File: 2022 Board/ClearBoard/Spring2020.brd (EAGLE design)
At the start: 100 x 80 mm, 18 parts, among them U1 TB67H401FTG(O,EL), U2 ABX00012, U3 V36SE05010NRFA

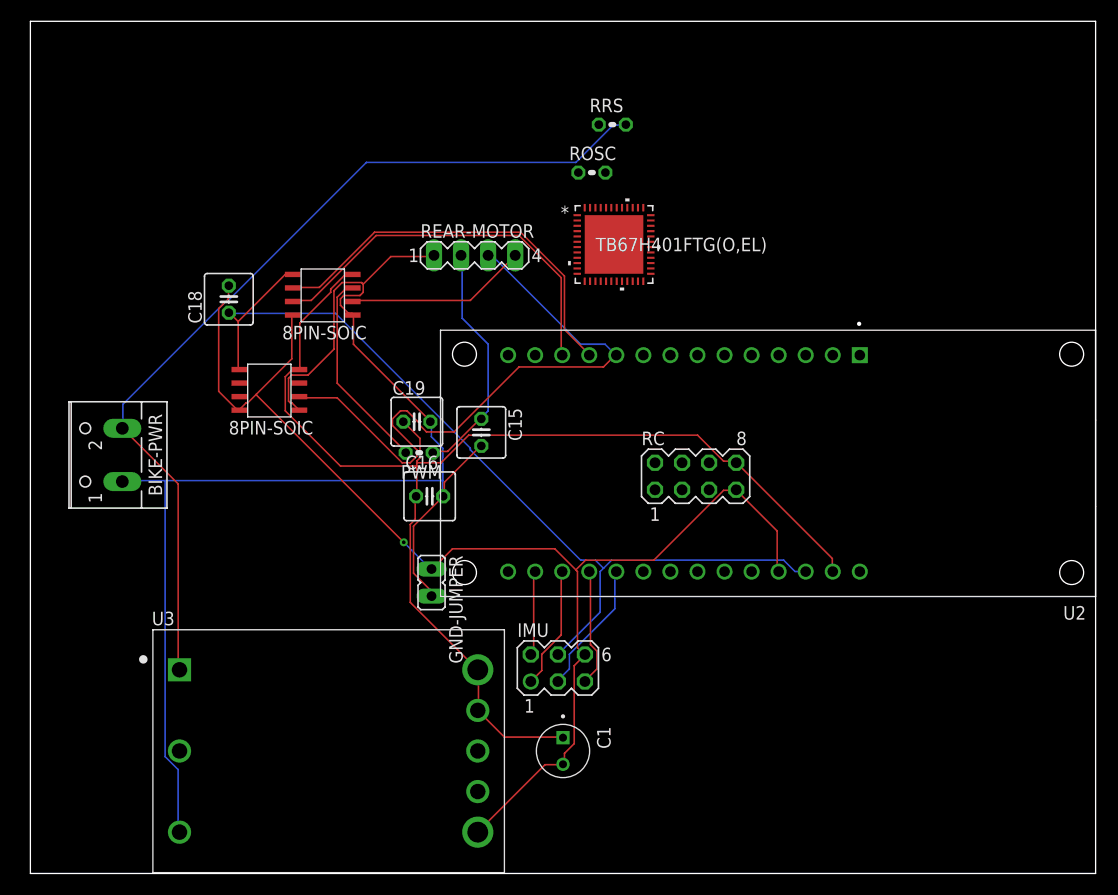
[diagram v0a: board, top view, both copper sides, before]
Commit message: Fixed a bunch of stuff
Routed most of the board
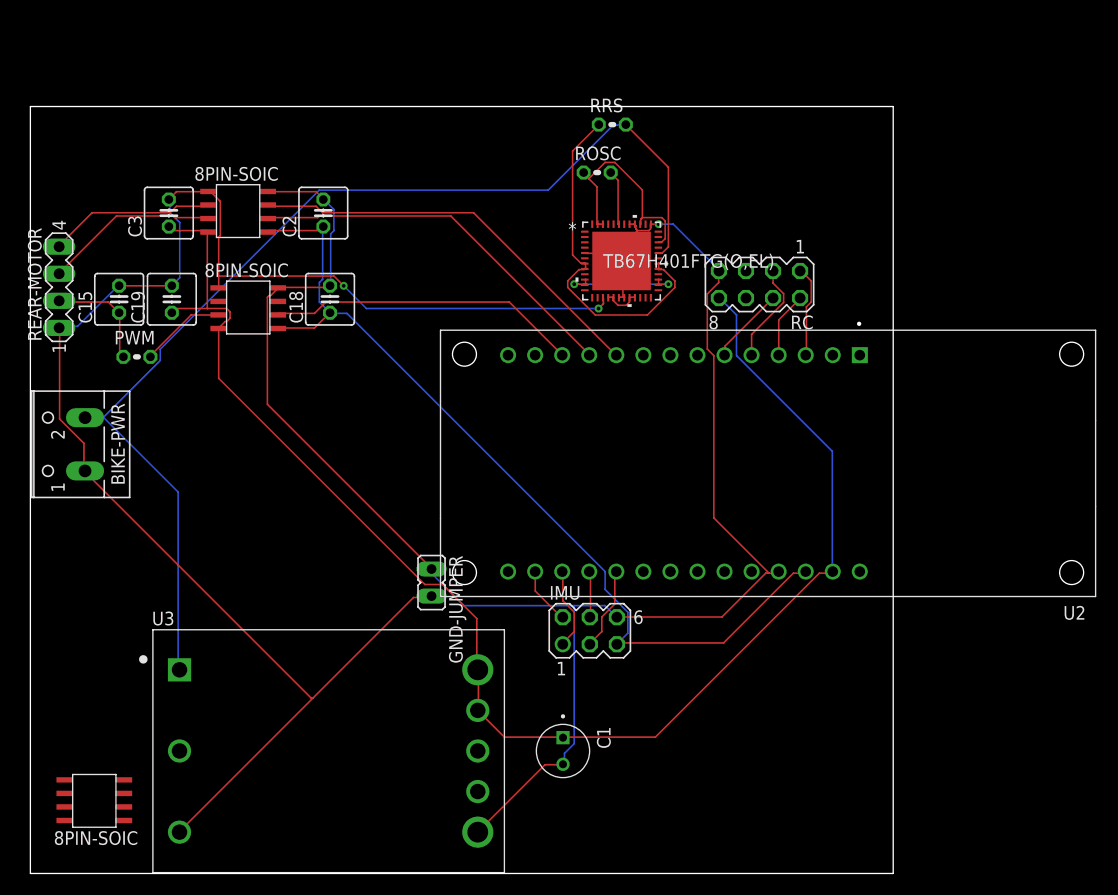
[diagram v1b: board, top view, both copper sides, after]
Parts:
- removed C16: (no value), resistor:C025-050X050
- added C2, C3: (no value), resistor:C025-050X050
- added U$3: IL-711, Spring2016Optoisolator:8PINSOIC
- U$2: value IL-711 -> IL-712
- U1: device mclr:P-VQFN48-0707-0P50-004_TOS -> Test:P-VQFN48-0707-0P50-004_TOS
- moved REAR-MOTOR 39.1 mm to (2.70, 55.0), turned to 90 degrees
- moved C15 36.2 mm to (8.33, 53.9), turned to 90 degrees
- moved PWM 28.0 mm to (10.0, 48.5), turned to 0 degrees
- moved C19 25.7 mm to (13.3, 53.9), turned to 90 degrees
- moved RC 19.0 mm to (68.5, 55.3), turned to 180 degrees
- moved U$2 17.7 mm to (19.5, 62.5), turned to 180 degrees
- moved C18 9.50 mm to (28.1, 53.9)
- moved U$7 7.02 mm to (20.4, 53.5), turned to 180 degrees
- moved IMU 4.61 mm to (52.5, 22.8)
- moved BIKE-PWR 3.64 mm to (3.86, 40.3)
- moved U1 1.70 mm to (55.5, 57.5)
- moved ROSC 0.50 mm to (53.2, 65.8)
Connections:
- new net GND1: U$3.4
- new net GND2: U$3.5
- new net N$2: U1.22
- new net VDD1: U$3.1
- new net VDD2: U$3.8
- net 3.3V: now also C2.1, IMU.5; no longer IMU.4
- net 5V: now also C3.1; no longer C16.1
- net BKGND: now also C3.2; no longer C16.2, U1.22
- net CH1: now also U2.3
- net CH2: now also U2.4
- net CH3: now also U2.5
- net CH4: now also U2.6
- net GND: now also C2.2
- net REAR-PWM: now also U2.12; no longer U2.11
- net REAR-TIMER: now also U$2.6; no longer U$7.6
- net REAR-TIMER-IN: now also U$2.3, U2.10; no longer U$7.3, U2.12
- net REVERSE: now also U$2.7; no longer U$2.6, U2.10
- net REVERSE_IN: now also U$2.2, U2.11; no longer U$2.3
- net SCK: now also IMU.4; no longer IMU.5
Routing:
- net GND: track 120.4 -> 169.3 mm
- net REVERSE: track 59.5 -> 16.4 mm
- net REVERSE_IN: track 0.00 -> 35.7 mm
- net RS: track 0.00 -> 33.5 mm
- net FVCC: track 0.00 -> 20.8 mm
- net 5V: track 116.7 -> 137.0 mm
- net BKPWR: track 85.3 -> 105.5 mm
- net BKGND: track 132.3 -> 150.8 mm, vias 0 -> 2
- net REAR-PWMOUT: track 22.6 -> 10.4 mm
- net F+: track 0.00 -> 12.0 mm, vias 0 -> 2
- net REAR-PWMR/SERVO2: track 19.1 -> 8.07 mm
- net CH3: track 0.00 -> 9.56 mm
- net CH1: track 0.00 -> 8.60 mm
- net REAR-PWM: track 37.7 -> 29.3 mm
- net CH4: track 0.00 -> 7.24 mm
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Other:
- board size 100 x 80 mm -> 81 x 72 mm
